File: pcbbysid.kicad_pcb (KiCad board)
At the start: 2 copper layers, 50.5 x 38.5 mm, 16 parts, among them Q1 NPN, SW1 SW_Push

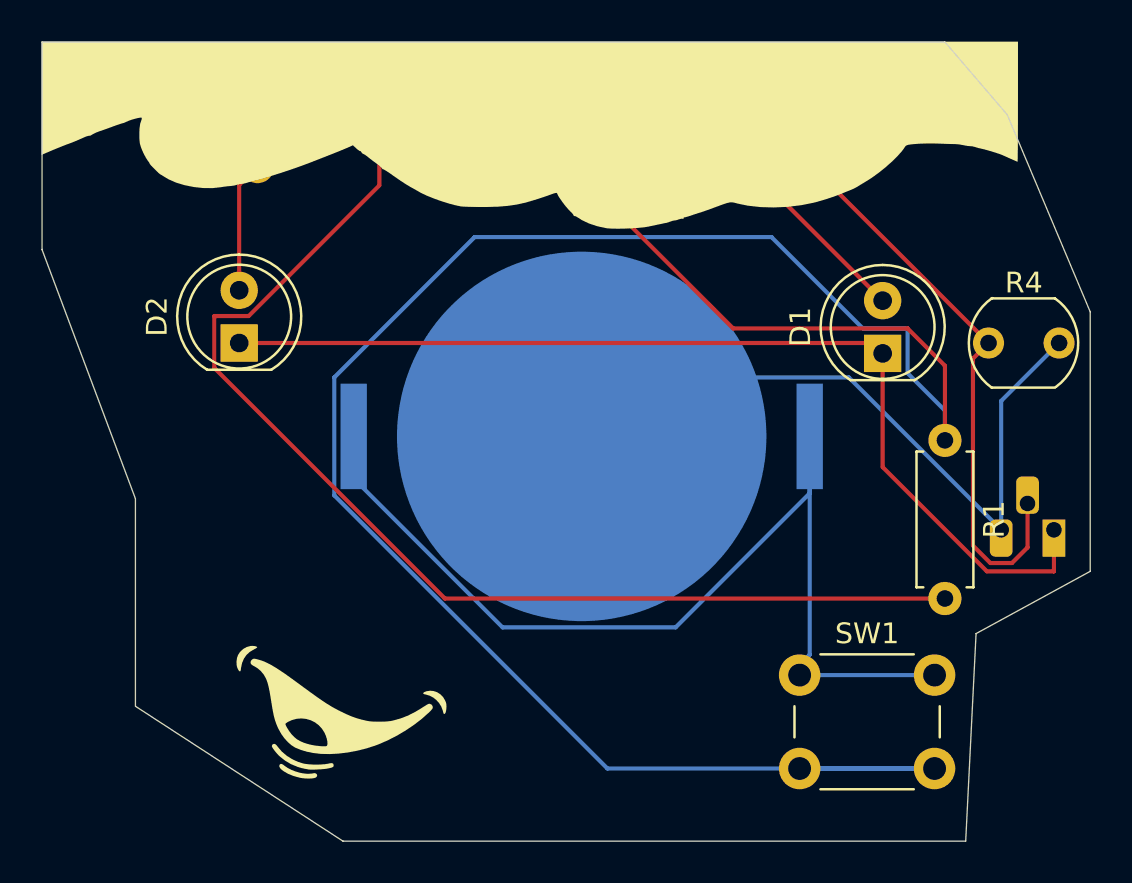
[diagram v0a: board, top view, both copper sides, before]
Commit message: Add files via upload
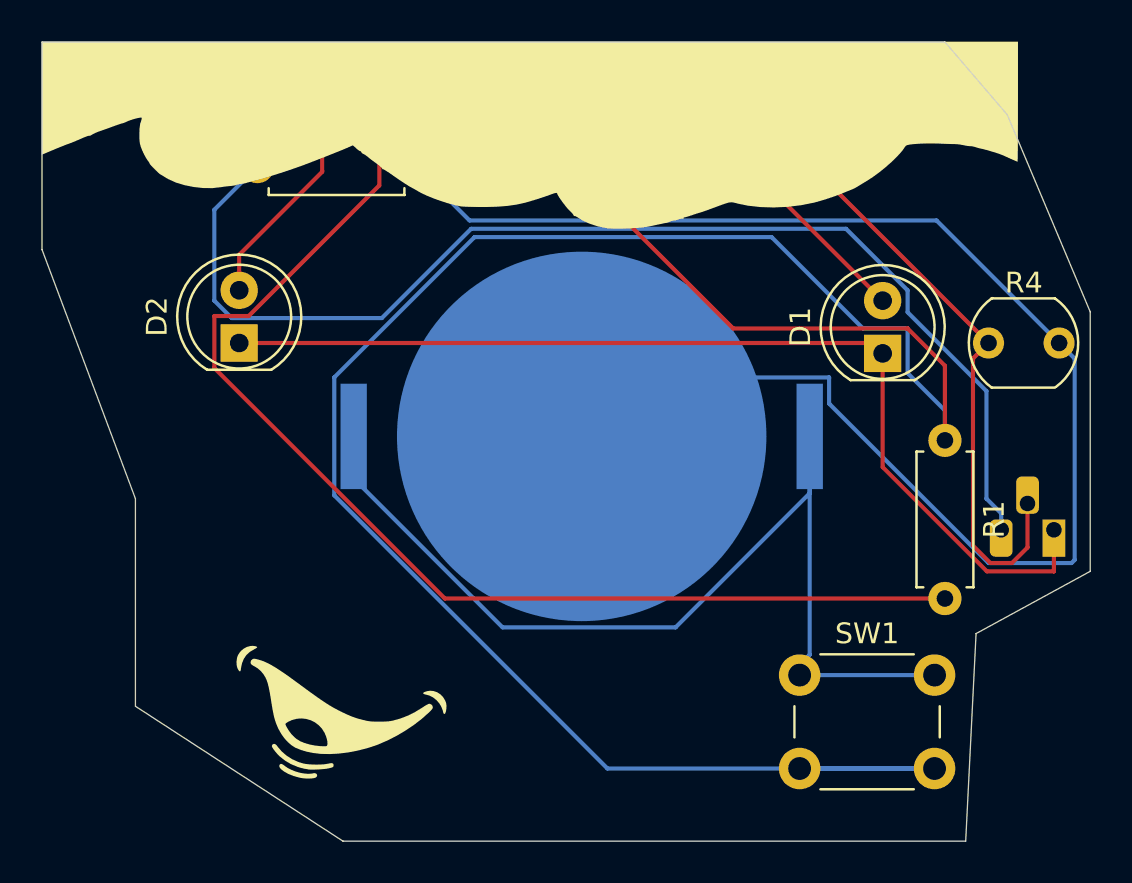
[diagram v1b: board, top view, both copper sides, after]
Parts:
- added R5: R, Resistor_THT:R_Axial_DIN0207_L6.3mm_D2.5mm_P7.62mm_Horizontal, F.Cu at (142.9, 64.0)
- moved R3 6.28 mm to (155.1, 59.8)
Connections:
- Q1 pad 3: Net-(BT1--) -> Net-(Q1-E)
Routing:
- net Net-(Q1-E): track 0.00 -> 57.5 mm
- net Net-(BT1--): track 34.6 -> 74.7 mm
- net Net-(D2-A): track 6.32 -> 13.1 mm
- net Net-(R1-Pad1): track 118.0 -> 115.9 mm
